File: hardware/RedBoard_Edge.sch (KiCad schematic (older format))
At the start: 72 parts, among them J1 CONN_025MM, J17 QWIIC_CONNECTORJS-1MM, J2 CONN_03X2SMT, J20 POWER_JACKSMD, J4 USB_MICRO-B_FEMALE-SMT, J5 CONN_04, J6 CONN_04, Q1 MOSFET_PCH-SI2309DS, Q2 MOSFET-NCH-BSS138, Q3 MOSFET-NCH-BSS138, U1 CH340GSMD, U2 V_REG_MIC52053.3V, U3 Standoff_Grounding, U4 ATMEGA328P_TQFP, U5 Standoff_Grounding, U6 V_REG_LM1117SOT223, Y1 RESONATOR-16MHZSMD_3.2X1.3, Y2 CRYSTAL-12MHZ\"

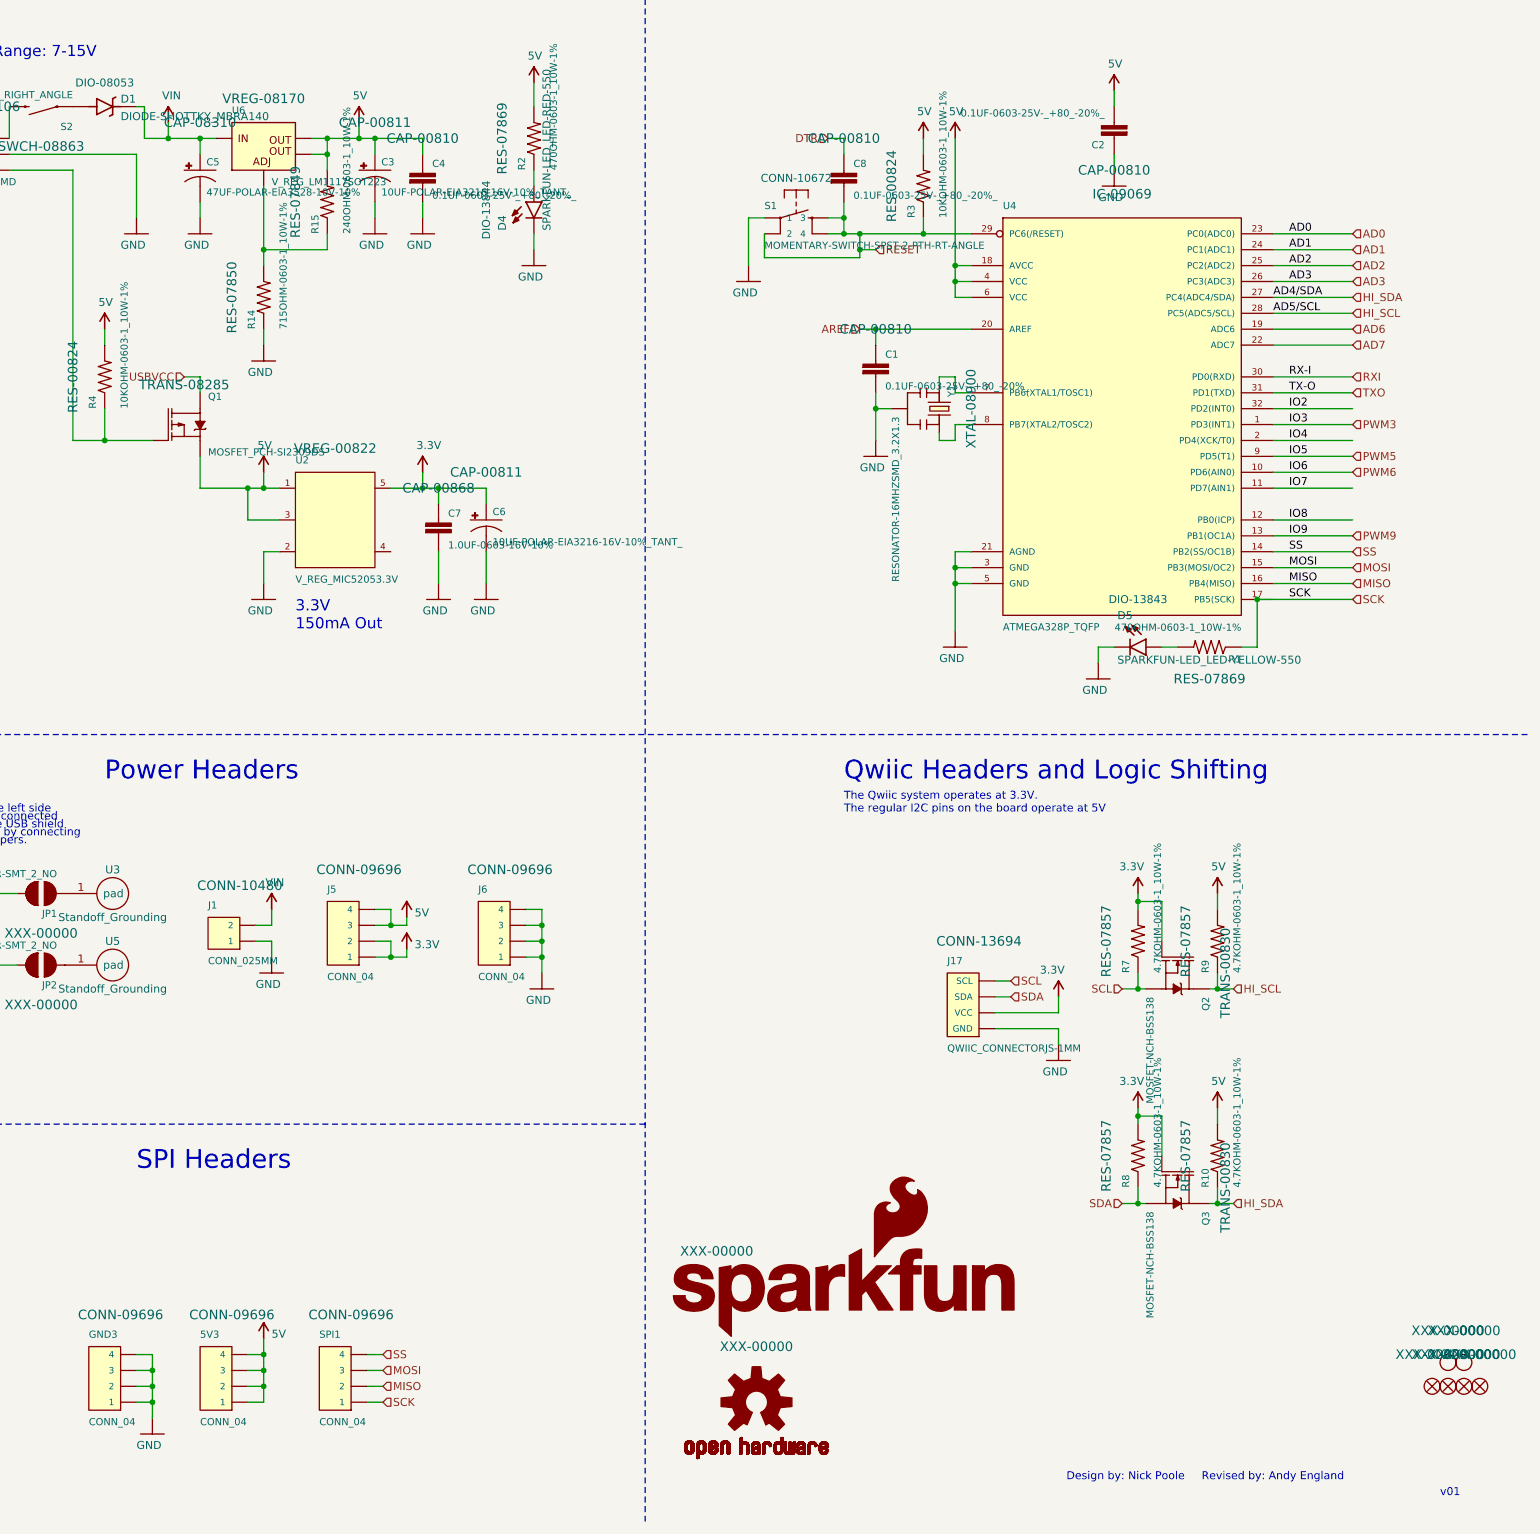
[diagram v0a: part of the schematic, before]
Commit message: v02
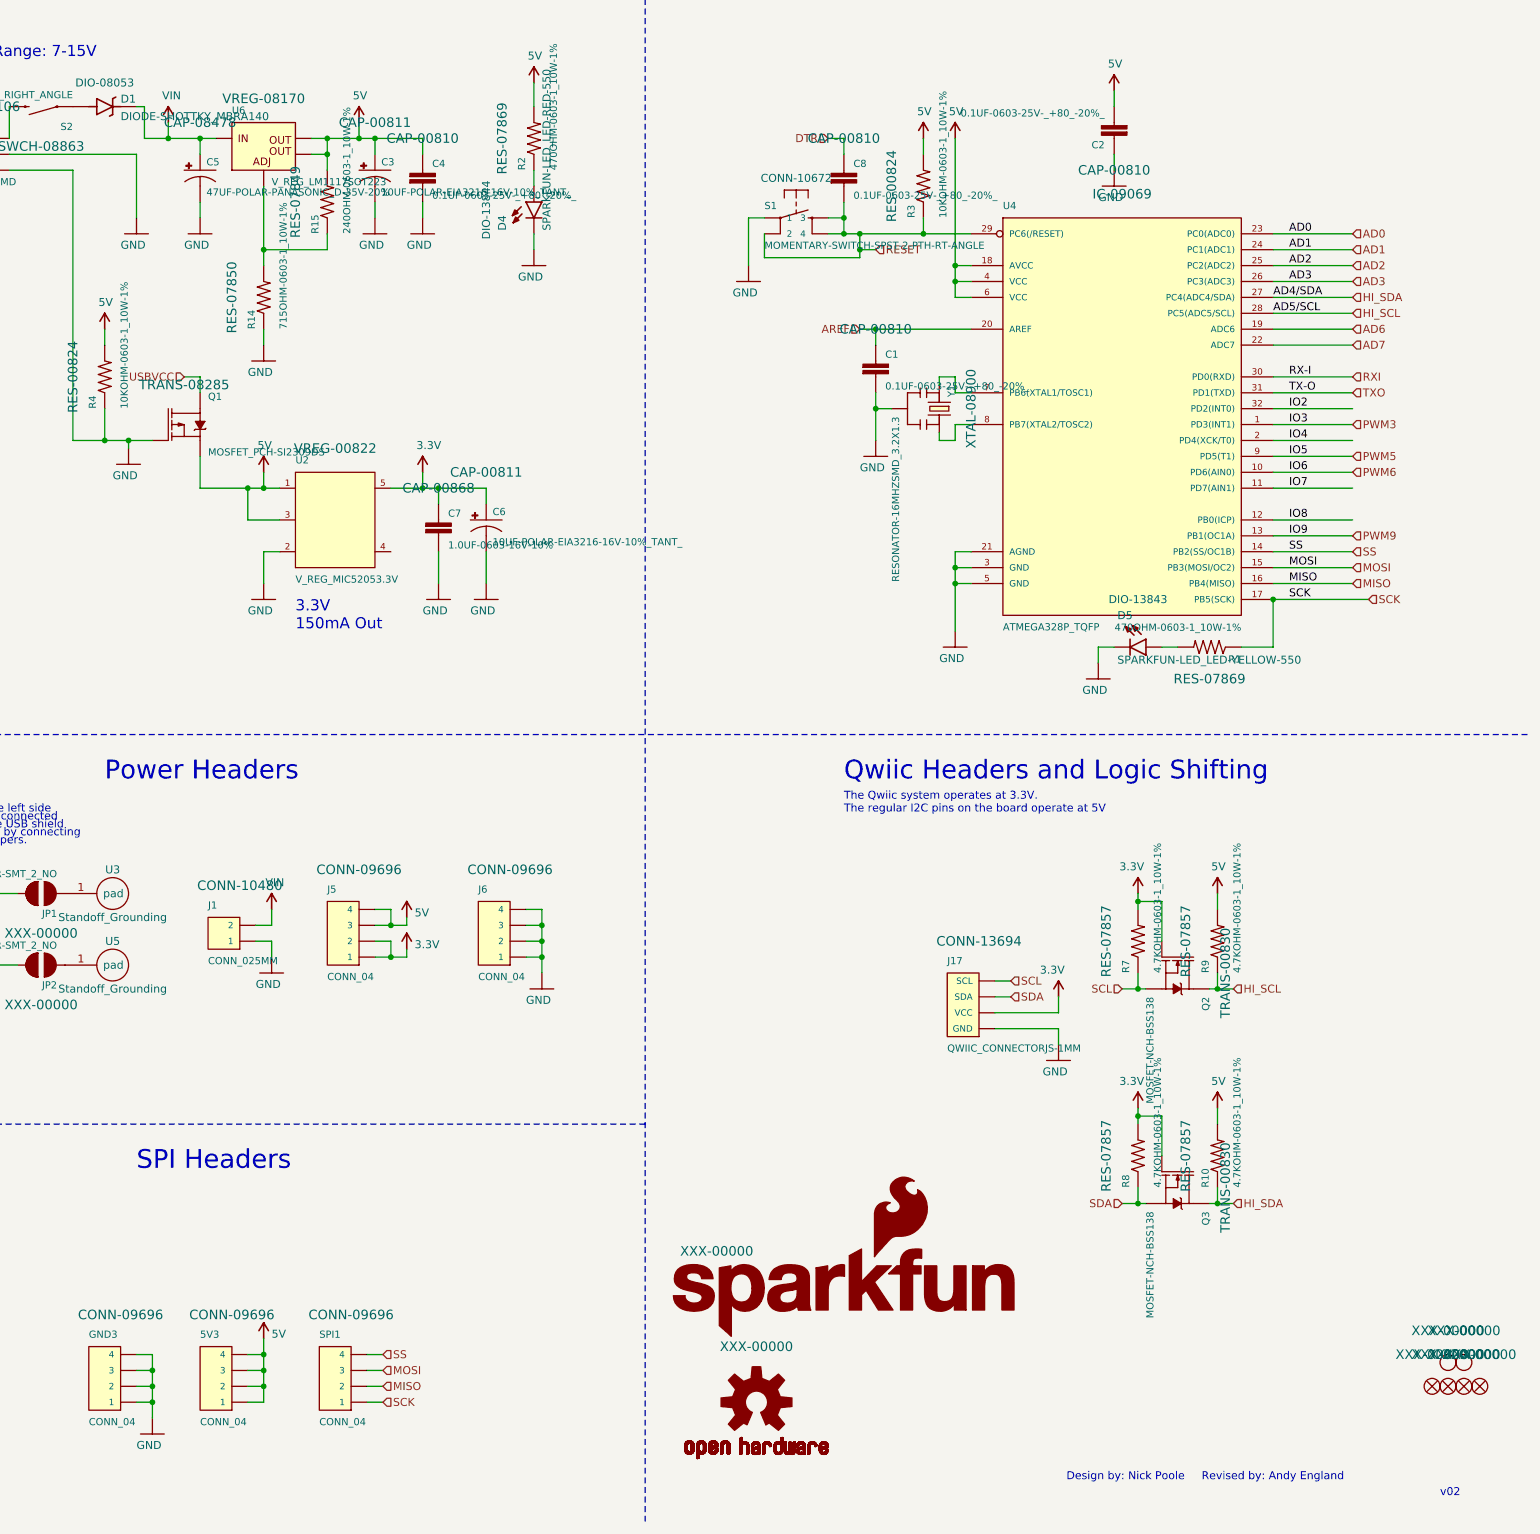
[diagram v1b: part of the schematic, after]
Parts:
- removed C5: 47UF-POLAR-EIA3528-10V-10%, symbol 47UF-POLAR-EIA3528-10V-10%
- added C5: 47UF-POLAR-PANASONIC_D-35V-20%, Capacitors:PANASONIC_D, symbol 47UF-POLAR-PANASONIC_D-35V-20%
- C1, C10, C11, C12, C2, C4, C7, C8, C9: footprint (none) -> Capacitors:0603
- C3, C6: footprint (none) -> Capacitors:EIA3216
- D1: footprint (none) -> Silicon-Standard:SMA-DIODE
- D2, D3, D4, D5: footprint (none) -> LED:LED_550_T1-.75_RT_ANG_PCB
- F1: footprint (none) -> Fuses:1206
- FD1, FD2, FD3, FD4: footprint (none) -> Aesthetics:FIDUCIAL-1X2
- H1, H2: footprint (none) -> Hardware:STAND-OFF
- J1: footprint SCREWTERMINAL-5MM-2 -> Connectors:SCREWTERMINAL-5MM-2
- J17: footprint (none) -> Connectors:1X04_1MM_RA
- J2: footprint (none) -> Connectors:2X3-NS
- J4: footprint (none) -> Connectors:USB-B-MICRO-SMD
- J5, J6, PWM1, SPI1: footprint (none) -> Connectors:1X04_NO_SILK
- JP1, JP2: footprint (none) -> Jumpers:SMT-JUMPER_2_NO_NO-SILK
- LOGO1: footprint SFE_LOGO_NAME_FLAME_.1 -> Aesthetics:SFE_LOGO_NAME_FLAME_.1
- LOGO2: footprint OSHW-LOGO-S -> Aesthetics:OSHW-LOGO-S
- Q1, Q2, Q3: footprint (none) -> Silicon-Standard:SOT23-3
- R1, R10, R14, R15, R2, R3, R4, R5, R6, R7, R8, R9: footprint (none) -> Resistors:0603
- S1: footprint (none) -> Switches:SWITCH TACTILE SPST-NO 0.05A 12V
- S2: footprint (none) -> Switches:RockerSwitch_RA
- U1: footprint (none) -> Silicon-Standard:SO16
- U2: footprint (none) -> Silicon-Standard:SOT23-5
- U3, U5: footprint (none) -> Hardware:STANDOFF_GROUNDING
- U4: footprint (none) -> Silicon-Standard:TQFP32-08
- U6: footprint (none) -> Silicon-Standard:SOT223
- Y1: footprint (none) -> Clocks:RESONATOR-SMD-3.2X1.3
- Y2: footprint CRYSTAL-SMD-5X3.2-4PAD -> Clocks:CRYSTAL-SMD-5X3.2-4PAD
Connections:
- net GND: now also J20.P$4 (GND), Q1.1 (G), R4.1, C5.-
- net SCK: now also U4.17 (PB5(SCK))
- net VIN: now also C5.+
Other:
- note added: "v02"
- note removed: "v01"
